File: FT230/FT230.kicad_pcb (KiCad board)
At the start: 2 copper layers, 20.5 x 10.4 mm, 22 parts, among them J1 USB_B_Micro, J2 Conn_01x04, J3 Conn_01x02, J4 Conn_01x02, U1 FT230XQ

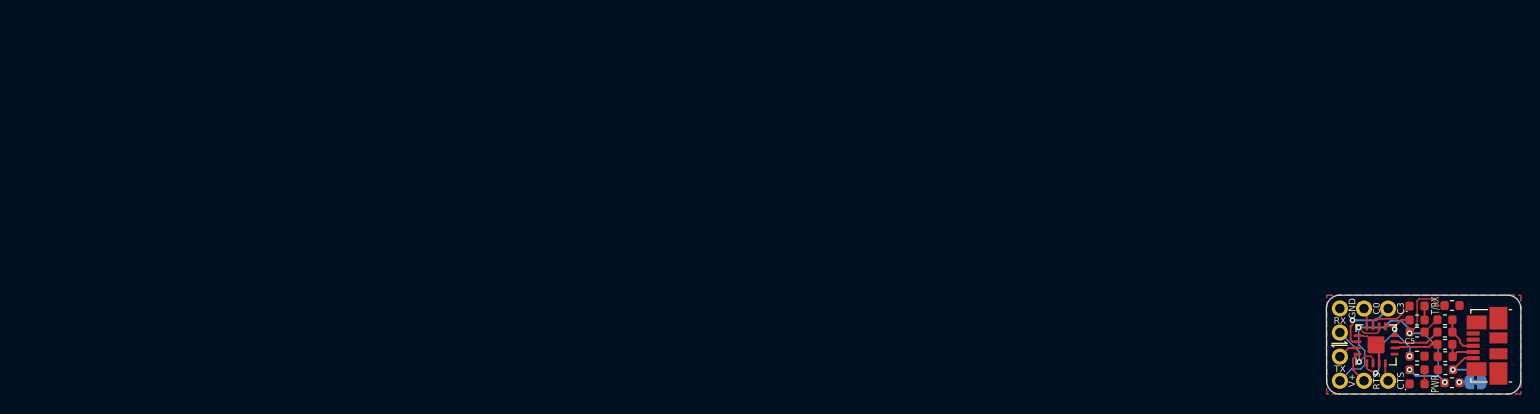
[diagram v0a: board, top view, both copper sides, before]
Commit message: Page Settings Updated
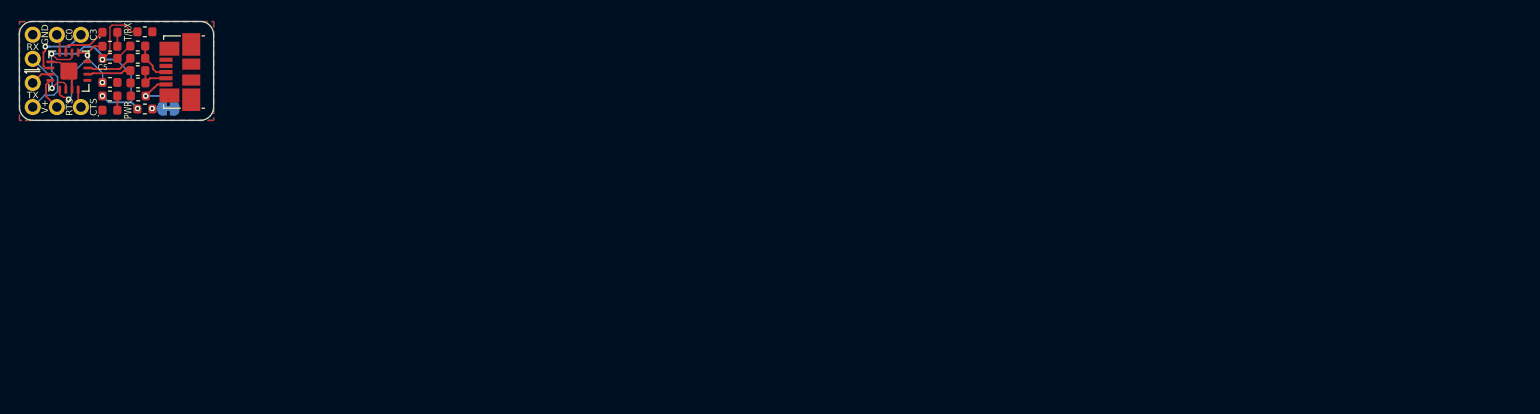
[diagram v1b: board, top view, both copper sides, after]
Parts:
- moved C1 140.7 mm to (69.5, 45.9)
- moved C2 140.7 mm to (69.5, 40.6)
- moved C3 140.7 mm to (69.5, 44.5)
- moved C4 140.7 mm to (70.2, 39.1)
- moved C5 140.7 mm to (66.6, 41.9)
- moved C6 140.7 mm to (66.5, 44.5)
- moved FB1 140.7 mm to (70.2, 47.2)
- moved G*** 140.7 mm to (67.5, 43.2)
- moved J1 140.7 mm to (73.9, 43.4)
- moved J2 140.7 mm to (58.4, 47.0)
- moved JP1 140.7 mm to (72.7, 47.2)
- moved PWR 140.7 mm to (66.5, 47.4)
- moved R1 140.7 mm to (69.5, 41.9)
- moved R2 140.7 mm to (69.5, 43.2)
- moved R3 140.7 mm to (66.5, 40.6)
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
